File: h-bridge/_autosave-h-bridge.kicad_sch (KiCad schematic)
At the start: 25 parts, among them M1 Motor_DC, Q1 IRF4905, Q2 IRLZ44N, Q3 IRF4905, Q4 IRLZ44N, Q5 2N2222, Q6 2N2222, Q7 IRF4905, Q8 2N2222, U1 74HC08

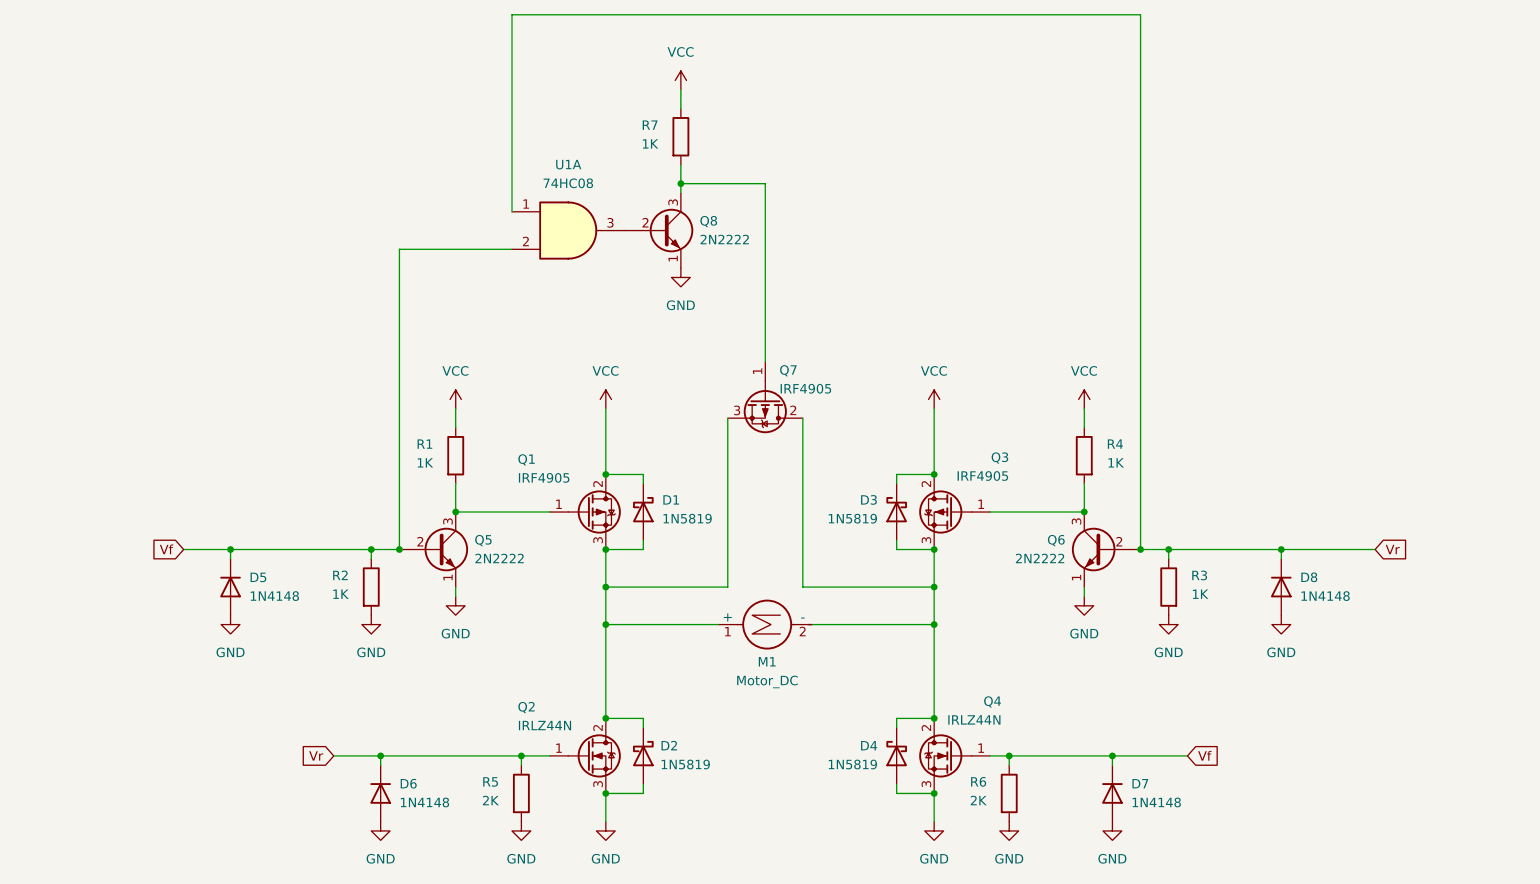
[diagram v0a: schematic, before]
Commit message: First POC
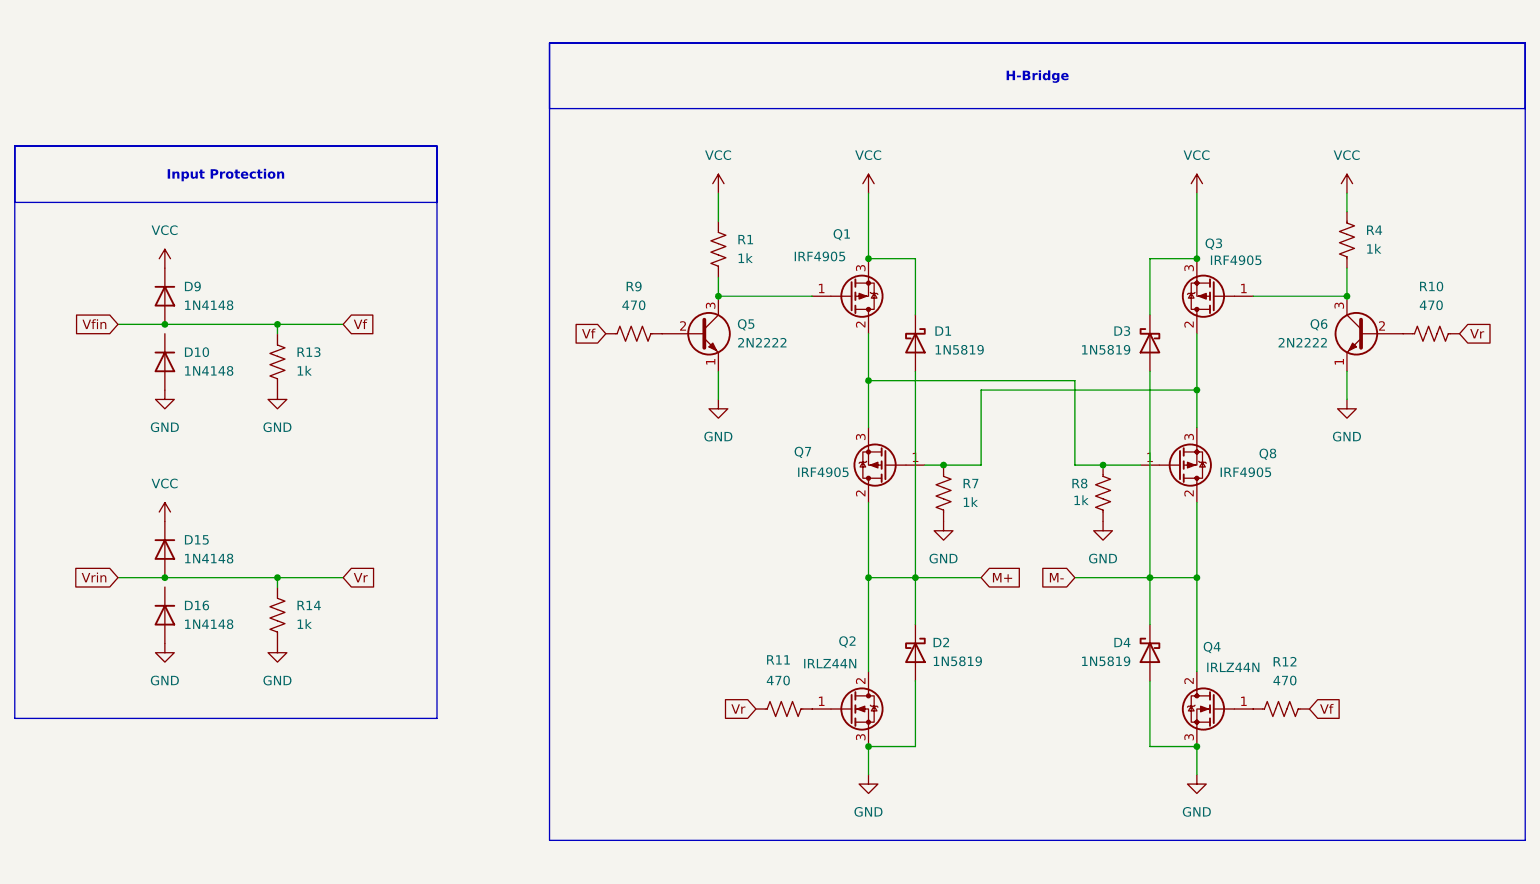
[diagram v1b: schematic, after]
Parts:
- removed D5, D6, D7, D8: 1N4148, Diode_THT:D_DO-35_SOD27_P7.62mm_Horizontal, symbol Diode:1N4148
- removed M1: Motor_DC, symbol Motor:Motor_DC
- removed Q8: 2N2222, Package_TO_SOT_THT:TO-39-3, symbol Transistor_BJT:2N2219
- removed R1, R2, R3, R4, R7: 1K, symbol Device:R
- removed R5, R6: 2K, symbol Device:R
- removed U1: 74HC08, symbol 74xx:74LS08
- added D10, D15, D16, D9: 1N4148, Diode_THT:D_DO-35_SOD27_P7.62mm_Horizontal, symbol Diode:1N4148
- added Q8: IRF4905, Package_TO_SOT_THT:TO-220-3_Vertical, symbol Transistor_FET:IRF4905
- added R1, R13, R14, R4, R7, R8: 1k, symbol Device:R_US
- added R10, R11, R12, R9: 470, symbol Device:R_US
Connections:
- net GND: now also D10.2 (A), D16.2 (A), R13.2, R14.2, R7.2, R8.2
- net VCC: now also Q1.3 (S), Q3.3 (S), D15.1 (K), D9.1 (K), R1.1, R4.1; no longer Q1.2 (D), Q3.2 (D)
- net Vf: now also D9.2 (A), R12.2, R13.1, R9.1; no longer Q4.1 (G), Q5.2 (B)
- net Vr: now also D15.2 (A), R10.2, R11.1, R14.1; no longer Q2.1 (G), Q6.2 (B)
- net at Q7.1 (G): now also Q3.2 (D), Q8.3 (S), R7.1
- net M-: now reaches D3.2 (A), D4.1 (K), Q4.2 (D)
- net M-: now also Q8.2 (D); no longer Q3.3 (S), Q7.2 (D)
- net M+: now reaches D1.2 (A), D2.1 (K), Q2.2 (D)
- net M+: now also Q7.2 (D); no longer Q1.3 (S), Q7.3 (S)
- net at Q3.1 (G), Q6.3 (C): now also R4.2
- net at Q1.1 (G), Q5.3 (C): now also R1.2
- new net: Q6.2 (B), R10.1
- new net: Q4.1 (G), R12.1
- new net: Q1.2 (D), Q7.3 (S), Q8.1 (G), R8.1
- new net: Q2.1 (G), R11.2
- new net: Q5.2 (B), R9.2
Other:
- moved on the sheet: D1, D2, D3, D4, Q1, Q2, Q3, Q4, Q5, Q6
